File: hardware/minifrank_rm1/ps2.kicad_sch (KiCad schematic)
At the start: 8 parts

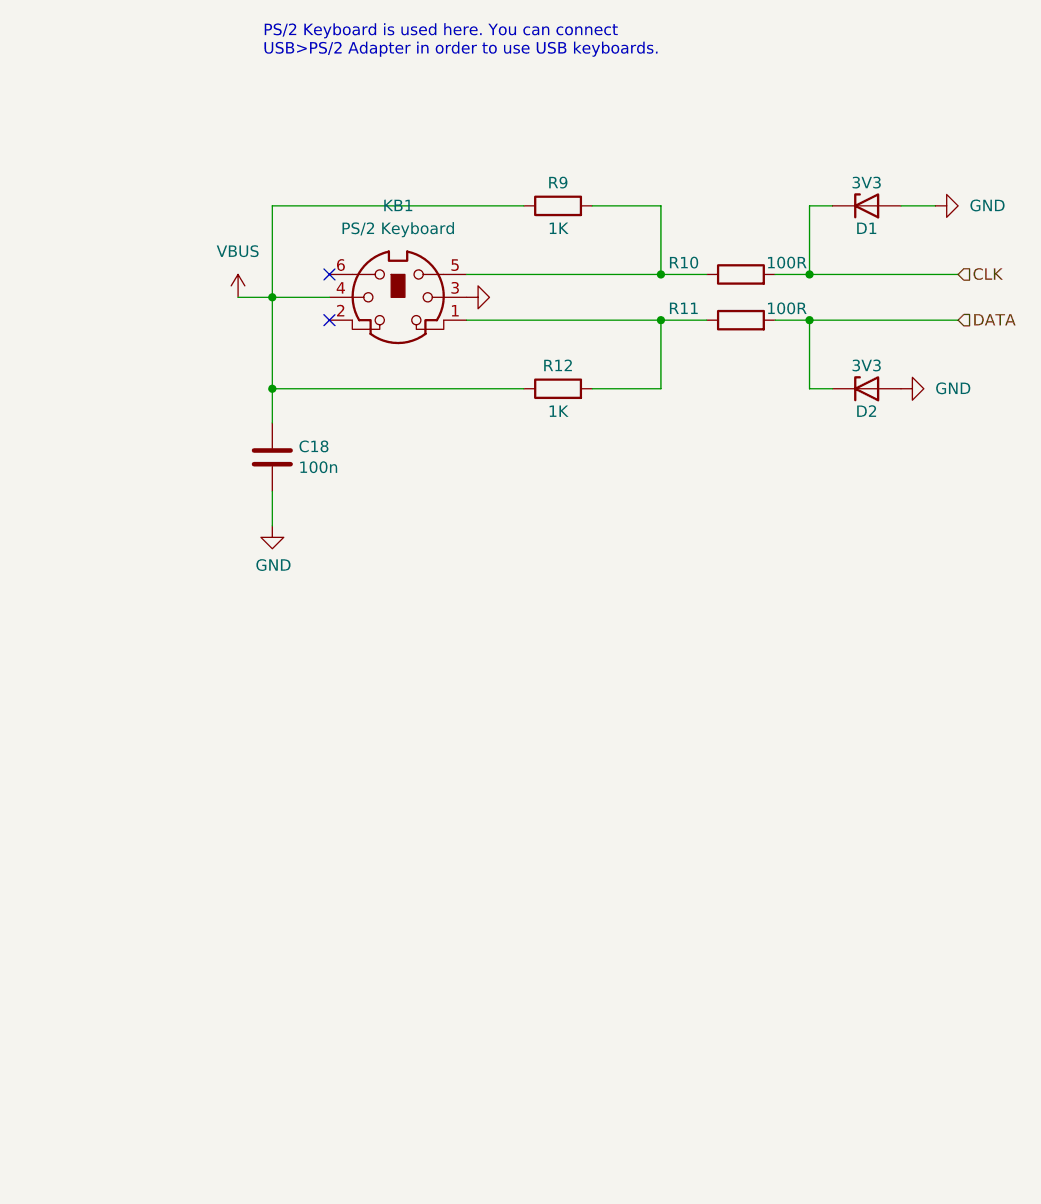
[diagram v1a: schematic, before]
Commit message: Minor updates
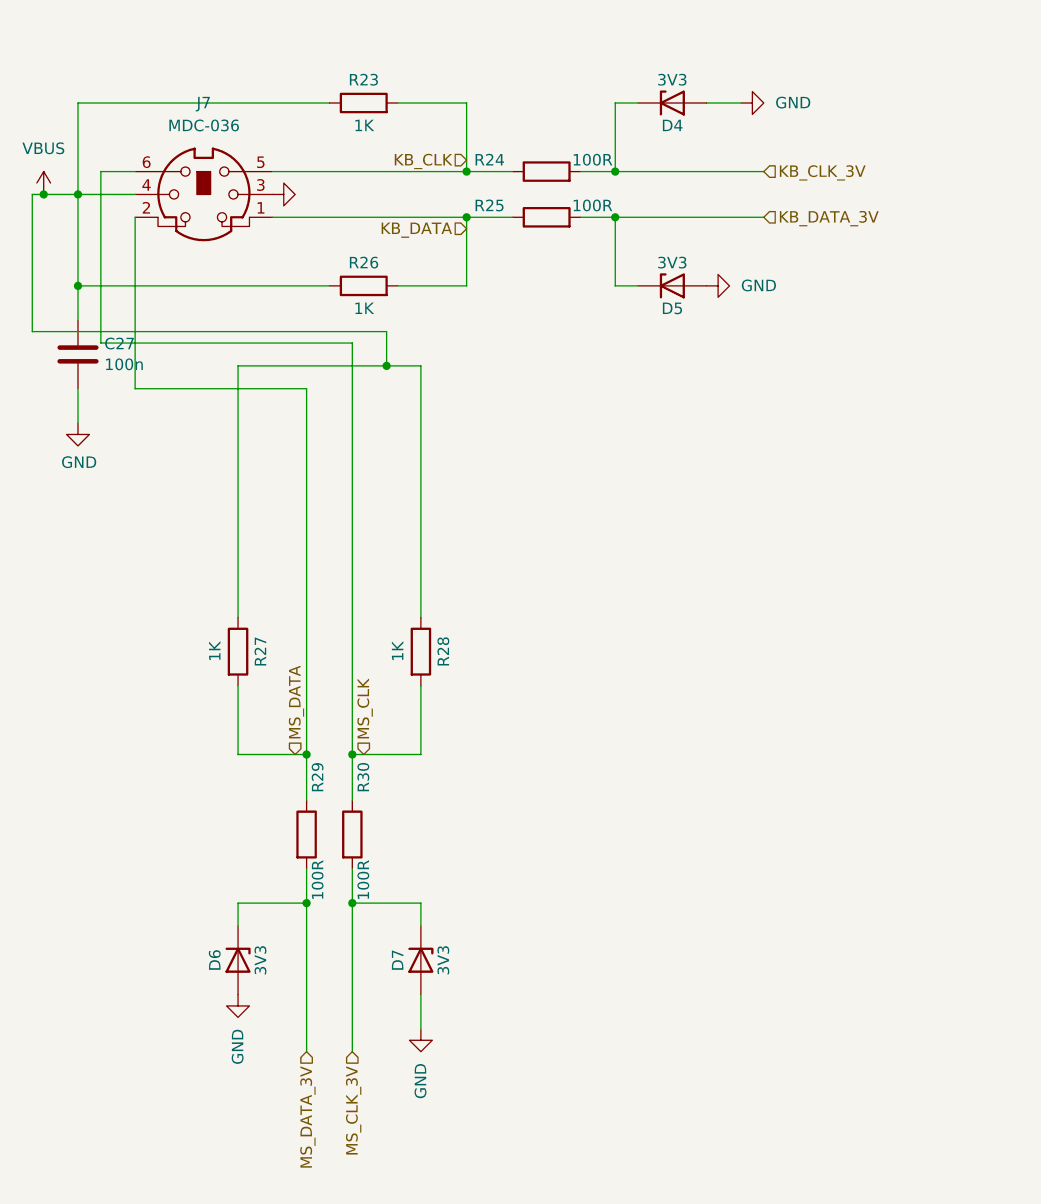
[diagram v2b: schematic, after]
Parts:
- added D6, D7: 3V3, FRANK:Diode (SOD-323), symbol Device:D_Zener
- added R27, R28: 1K, FRANK:Resistor (0805), symbol Device:R
- added R29, R30: 100R, FRANK:Resistor (0805), symbol Device:R
- D4: renamed from D1; AliExpress https://www.aliexpress.com/item/32997486634.html -> https://www.aliexpress.com/item/1005006143480992.html
- D5: renamed from D2; AliExpress https://www.aliexpress.com/item/32997486634.html -> https://www.aliexpress.com/item/1005006143480992.html
- J7: renamed from KB1; value PS/2 Keyboard -> MDC-036
- renumbered C18 to C27, R9 to R23, R10 to R24, R11 to R25, R12 to R26
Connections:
- net GND: now also D6.2 (A), D7.2 (A)
- net VBUS: now also R27.1, R28.1
- net KB_DATA: now reaches J7.1, R25.1, R26.2
- net KB_CLK: now reaches J7.5, R23.2, R24.1
- net MS_DATA: now reaches J7.2
- net MS_DATA: now also R27.2, R29.1
- net MS_CLK: now reaches J7.6
- net MS_CLK: now also R28.2, R30.1
- net CLK renamed KB_CLK_3V
- net DATA renamed KB_DATA_3V
- new net MS_CLK_3V: D7.1 (K), R30.2
- new net MS_DATA_3V: D6.1 (K), R29.2
- no-connect marks 2 -> 0
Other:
- note removed: "PS/2 Keyboard is used here. You can connect USB>PS/2 Adapter in order to use USB keyboards."
- moved on the sheet: C27, D4, D5, J7, R23, R24, R25, R26
